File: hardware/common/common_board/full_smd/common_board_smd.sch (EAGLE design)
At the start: 32 parts, among them U1 ATMEGA328P

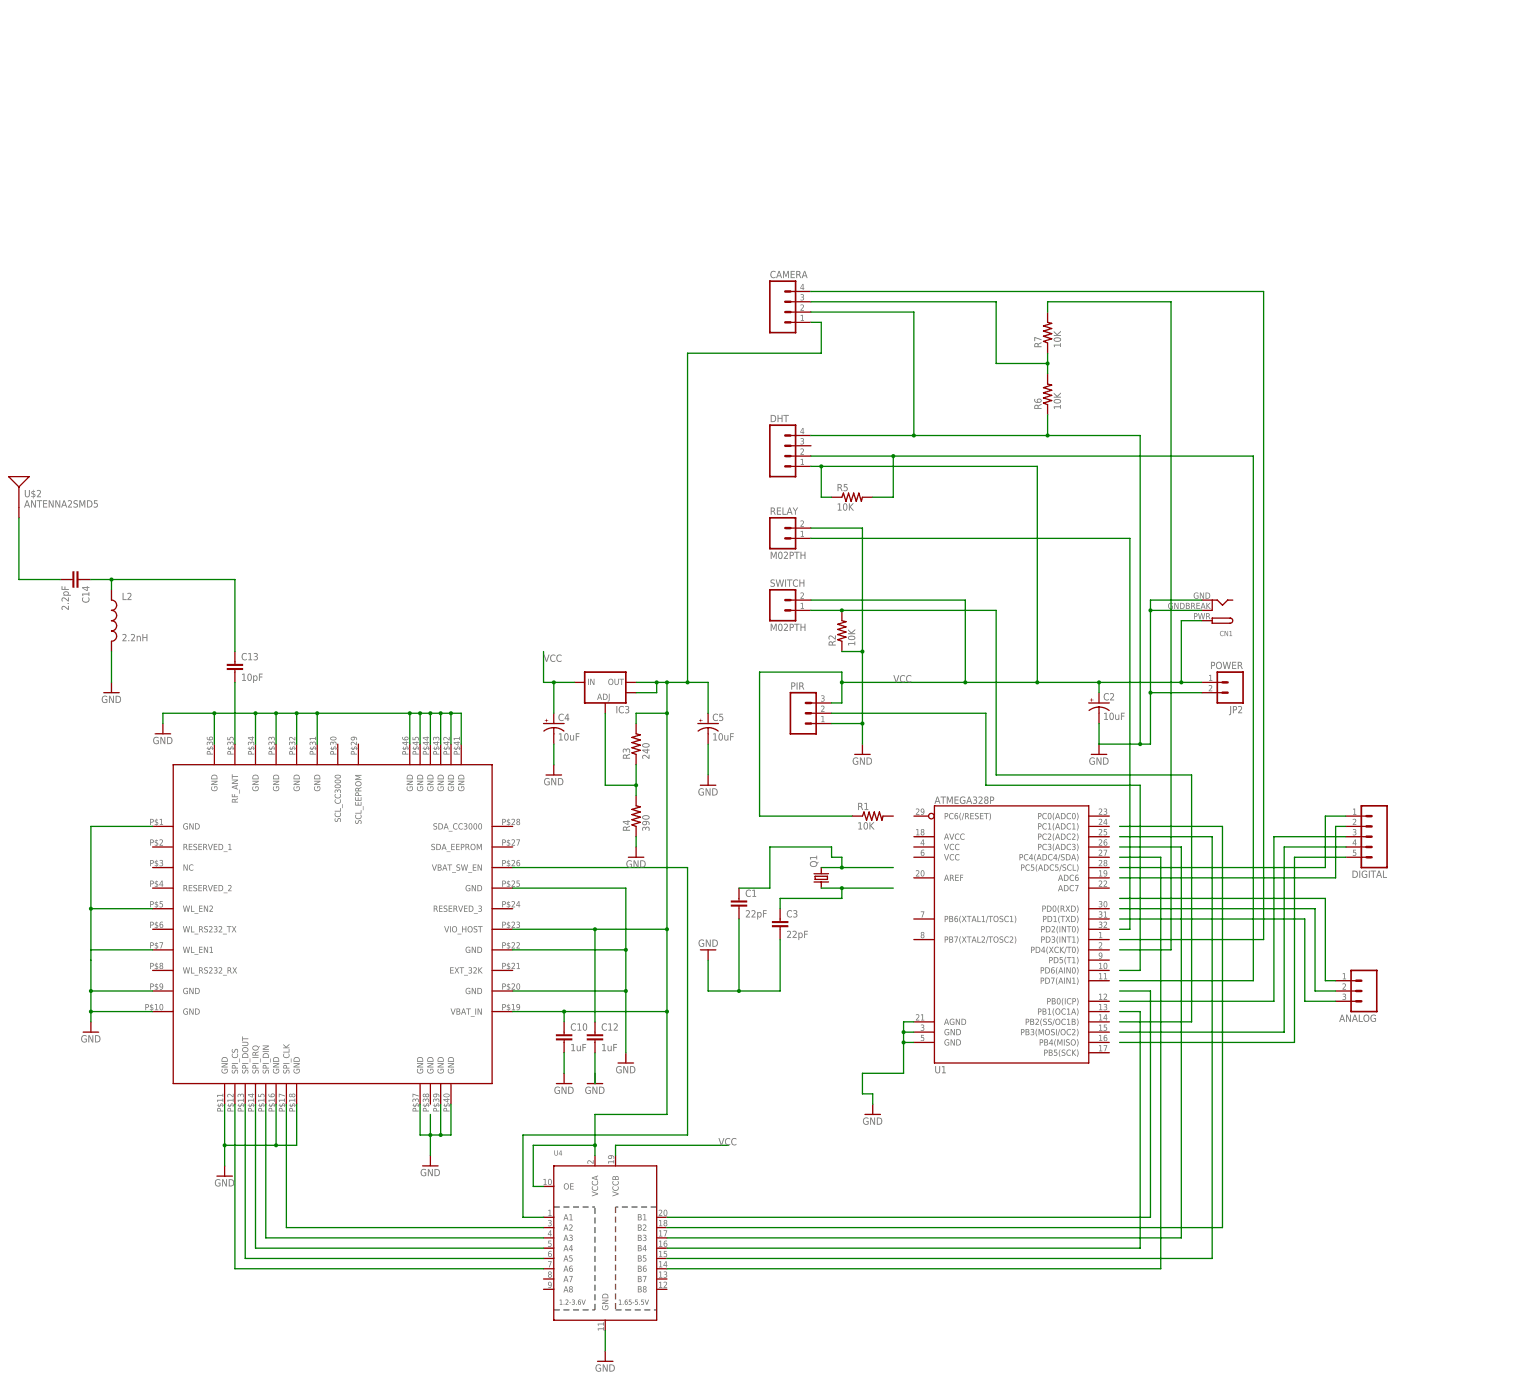
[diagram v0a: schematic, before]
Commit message: repo cleanup
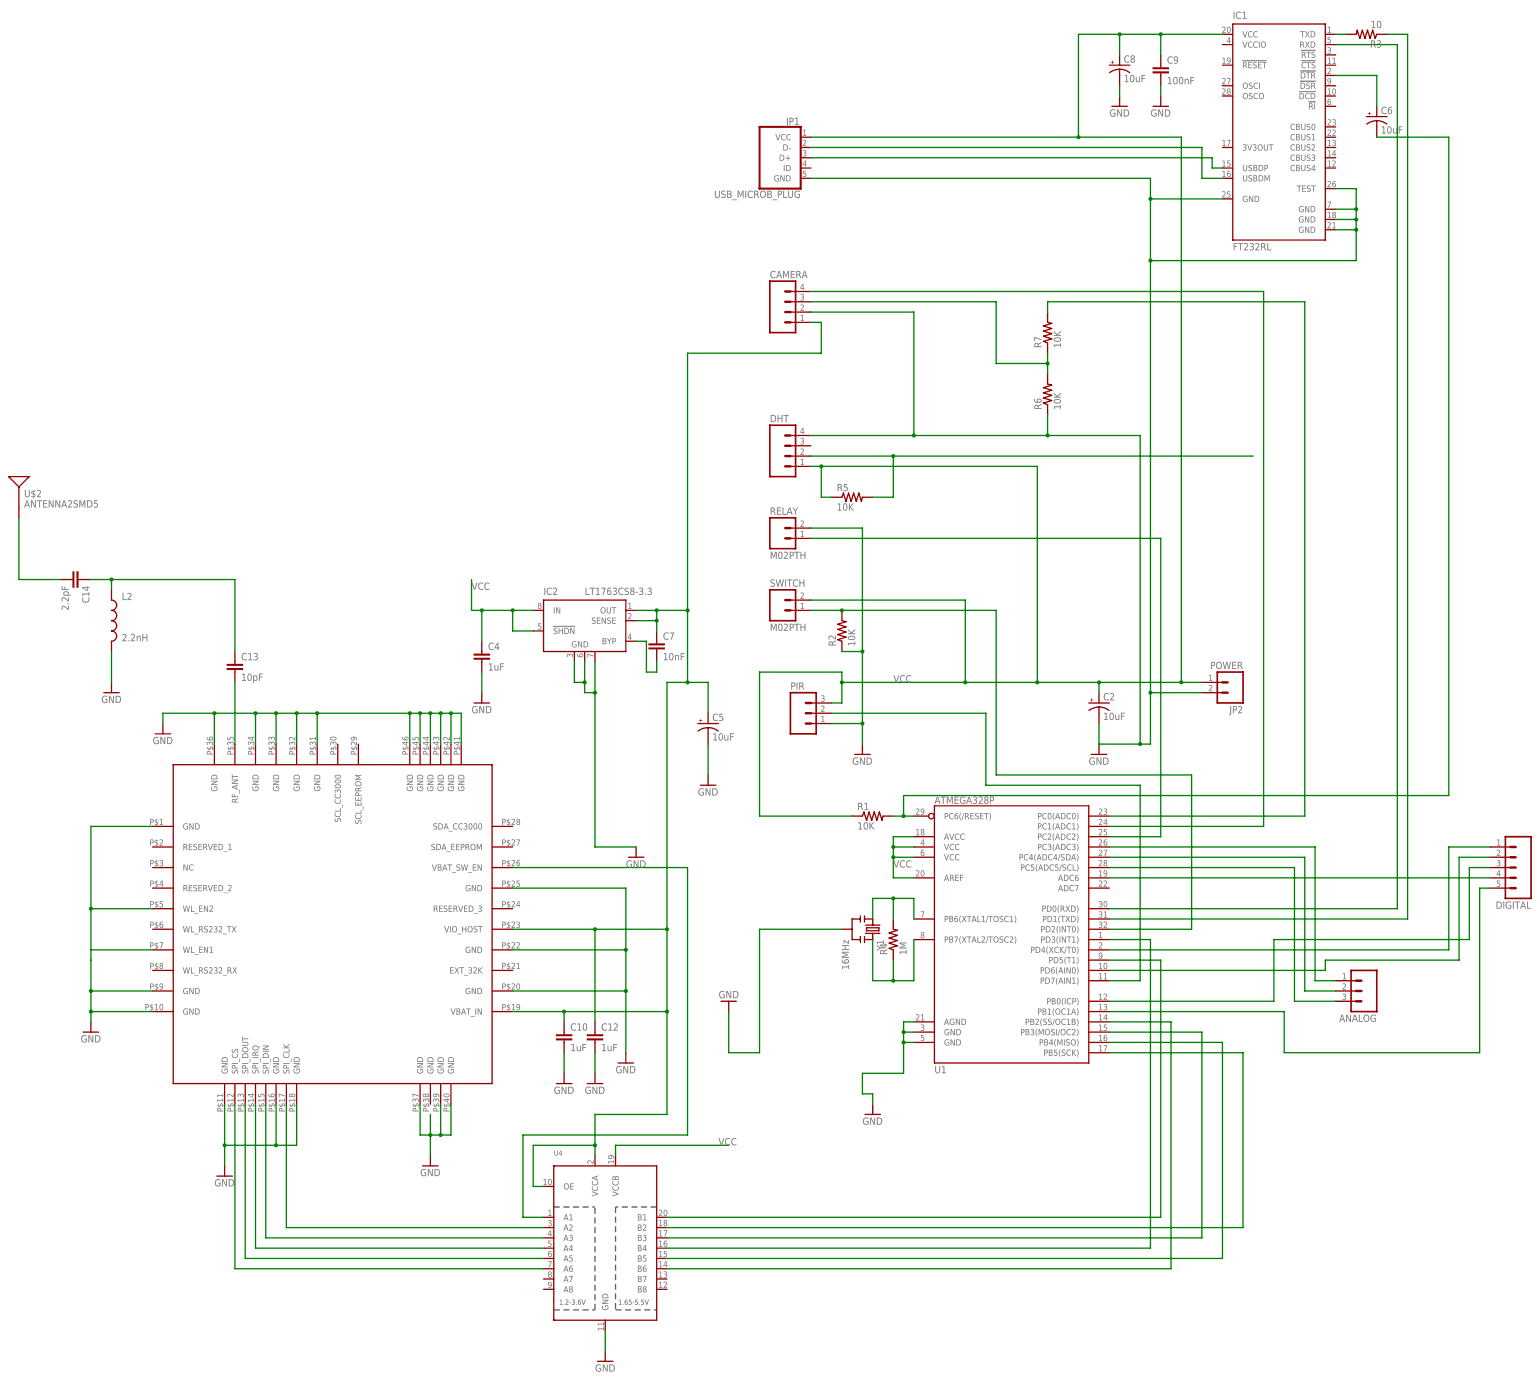
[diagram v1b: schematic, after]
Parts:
- removed C1, C3: 22pF, SparkFun-Passives:CAP0805
- removed CN1: (no value), adafruit:DCBARRELPTH
- removed IC3: (no value), SparkFun-PowerIC:V_REG_LM1117SOT223
- removed Q1: (no value), adafruit:CRYSTALHC49U-V
- added C6, C8: 10uF, SparkFun-Passives:CAP_POL1206
- added C7: 10nF, SparkFun-Capacitors:CAP0805
- added C9: 100nF, SparkFun-Capacitors:CAP0805
- added IC1: FT232RL, ftdichip:FT232RL
- added IC2: LT1763CS8-3.3, linear-technology:LT1763CS8-3.3
- added JP1: USB_MICROB_PLUG, SparkFun-Connectors:USB_MICROB_PLUG
- added Y1: 16MHz, SparkFun-FreqCtrl:RESONATOR16MHZ
- C4: value 10uF -> 1uF; device SparkFun-Passives:CAP_POL3528 -> SparkFun-Capacitors:CAP0805
- R3: value 240 -> 10; device SparkFun-Resistors:RESISTOR0805-RES -> SparkFun-Passives:RESISTOR0805-RES
- R4: value 390 -> 1M; device SparkFun-Resistors:RESISTOR0805-RES -> SparkFun-Resistors:RESISTOR0603-RES
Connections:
- removed net N$7: C12.2
- removed net XTAL2: C1.1, Q1.2
- new net N$3: C6.-, R1.2, U1.PC6(/RESET)
- new net N$36: DIGITAL.5, U1.PB1(OC1A)
- new net N$37: DIGITAL.3, U1.PB0(ICP)
- new net N$38: DIGITAL.1, U1.PD4(XCK/T0)
- new net N$39: DIGITAL.2, U1.PD6(AIN0)
- new net N$40: DIGITAL.4, U1.ADC6
- new net N$41: R4.1, U1.PB7(XTAL2/TOSC2), Y1.3
- new net N$42: C7.2, IC2.BYP
- net GND: now also C12.2, C4.2, C8.-, C9.2, IC1.GND, IC1.GND@1, IC1.GND@2, IC1.GND@A, IC1.TEST, IC2.GND@1, IC2.GND@2, IC2.GND@3, JP1.GND, Y1.2; no longer C1.2, C3.2, C4.-, CN1.GND, CN1.GNDBREAK, R4.1
- net N$1: now also U1.PD5(T1)
- net N$15: now also IC1.TXD, R3.2; no longer IC3.ADJ, R3.1, R4.2
- net N$19: now also U1.PB4(MISO)
- net N$2: now also U1.PD3(INT1)
- net N$20: now also U1.PB3(MOSI/OC2)
- net N$21: now also U1.PD2(INT0)
- net N$23: now also U1.PC2(ADC2)
- net N$25: now also U1.PC0(ADC0)
- net N$26: now also U1.PD7(AIN1)
- net N$27: now also U1.PC1(ADC1)
- net N$28: now also IC1.USBDP, JP1.D+; no longer ANALOG.3
- net N$29: now also IC1.USBDM, JP1.D-; no longer ANALOG.2
- net N$30: now also R3.1, U1.PD1(TXD); no longer ANALOG.1
- net N$31: now also IC1.RXD, U1.PD0(RXD); no longer DIGITAL.5
- net N$32: now also C6.+, IC1.!DTR; no longer DIGITAL.4
- net N$33: now also ANALOG.1, U1.PC3(ADC3); no longer DIGITAL.3
- net N$34: now also ANALOG.2, U1.PC4(ADC4/SDA); no longer DIGITAL.2
- net N$35: now also ANALOG.3, U1.PC5(ADC5/SCL); no longer DIGITAL.1
- net N$4: now also R4.2, U1.PB6(XTAL1/TOSC1), Y1.1; no longer C3.1, Q1.1
- net N$5: now also U1.PB5(SCK)
- net N$6: now also U1.PB2(SS/OC1B)
- net N$8: now also C7.1, IC2.OUT, IC2.SENSE; no longer IC3.OUT, IC3.OUT@1, R3.2
- net VCC: now also C4.1, C8.+, C9.1, IC1.VCC, IC2.!SHDN, IC2.IN, JP1.VCC, U1.AREF, U1.AVCC, U1.VCC@1, U1.VCC@2; no longer C4.+, CN1.PWR, IC3.IN
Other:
- moved on the sheet: DIGITAL, R3, R4
